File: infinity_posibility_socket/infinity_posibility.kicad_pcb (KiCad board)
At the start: 2 copper layers, 94 x 94 mm, 375 parts, among them SW1 SW_PUSH, SW10 SW_PUSH, SW11 SW_PUSH, SW12 SW_PUSH, SW13 SW_PUSH, SW14 SW_PUSH, SW15 SW_PUSH, SW16 SW_PUSH, SW17 SW_PUSH, SW18 SW_PUSH, SW19 SW_PUSH, SW2 SW_PUSH, SW20 SW_PUSH, SW21 SW_PUSH, SW22 SW_PUSH, SW23 SW_PUSH, SW24 SW_PUSH, SW25 SW_PUSH, SW3 SW_PUSH, SW4 SW_PUSH, SW5 SW_PUSH, SW6 SW_PUSH, SW7 SW_PUSH, SW8 SW_PUSH, SW9 SW_PUSH

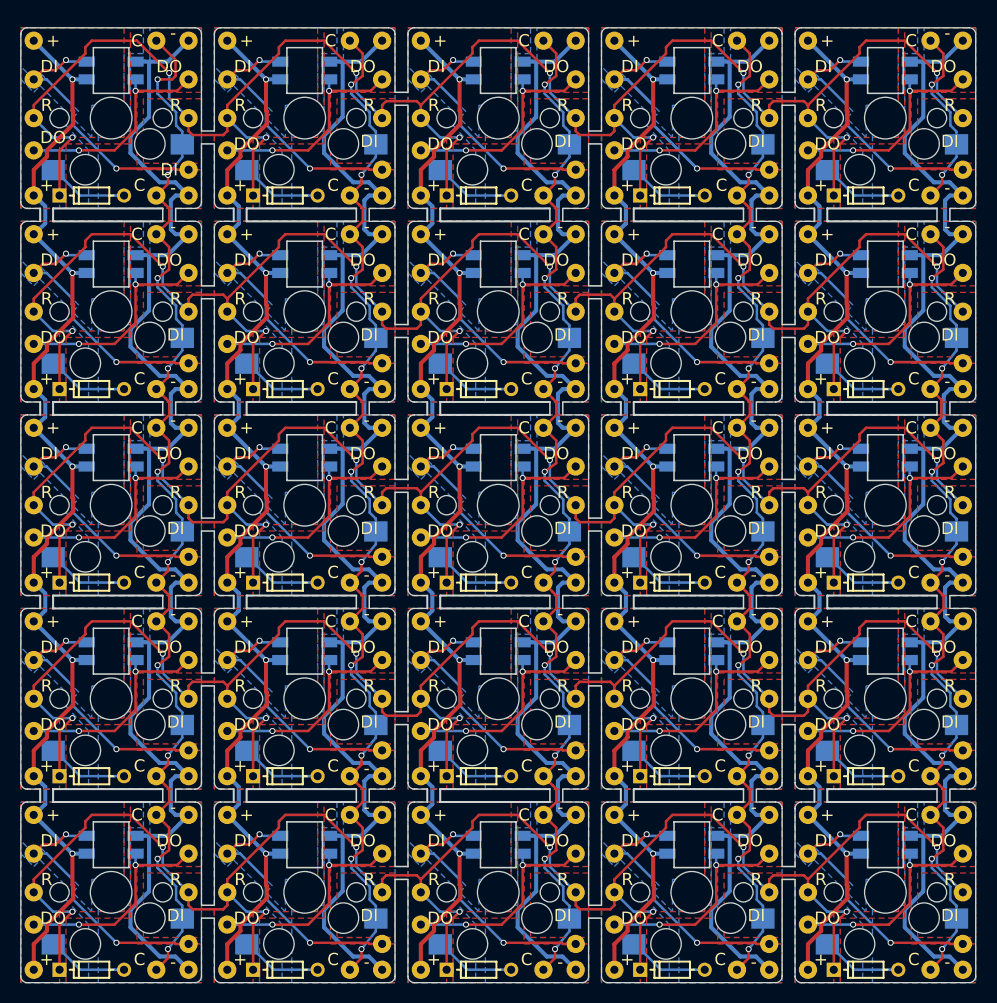
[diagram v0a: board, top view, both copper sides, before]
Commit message: renew
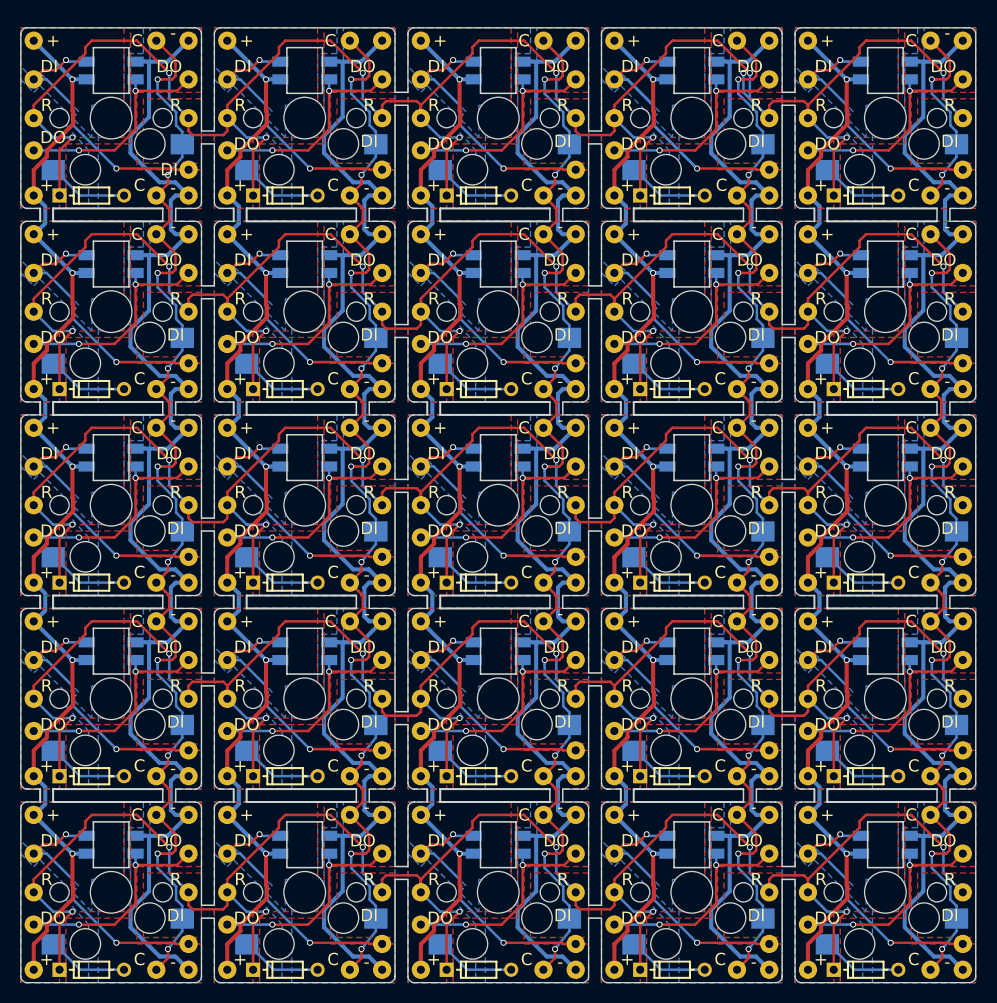
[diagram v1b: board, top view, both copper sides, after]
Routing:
- net /ROW0: track 197.7 -> 207.2 mm, vias 10 -> 11
- net /COL2: track 111.0 -> 117.3 mm
- net /COL4: track 105.9 -> 112.3 mm
- net /COL1: track 111.0 -> 117.3 mm
- net /COL3: track 111.0 -> 117.3 mm
- net /COL0: track 112.2 -> 117.3 mm
- net /ROW2: track 197.3 -> 201.7 mm
- net /ROW3: track 197.3 -> 201.7 mm
- net /ROW4: track 197.3 -> 201.7 mm
- net /ROW1: track 197.3 -> 201.7 mm
